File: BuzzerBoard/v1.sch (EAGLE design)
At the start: 7 parts, among them U1 LM386MX-1/NOPB

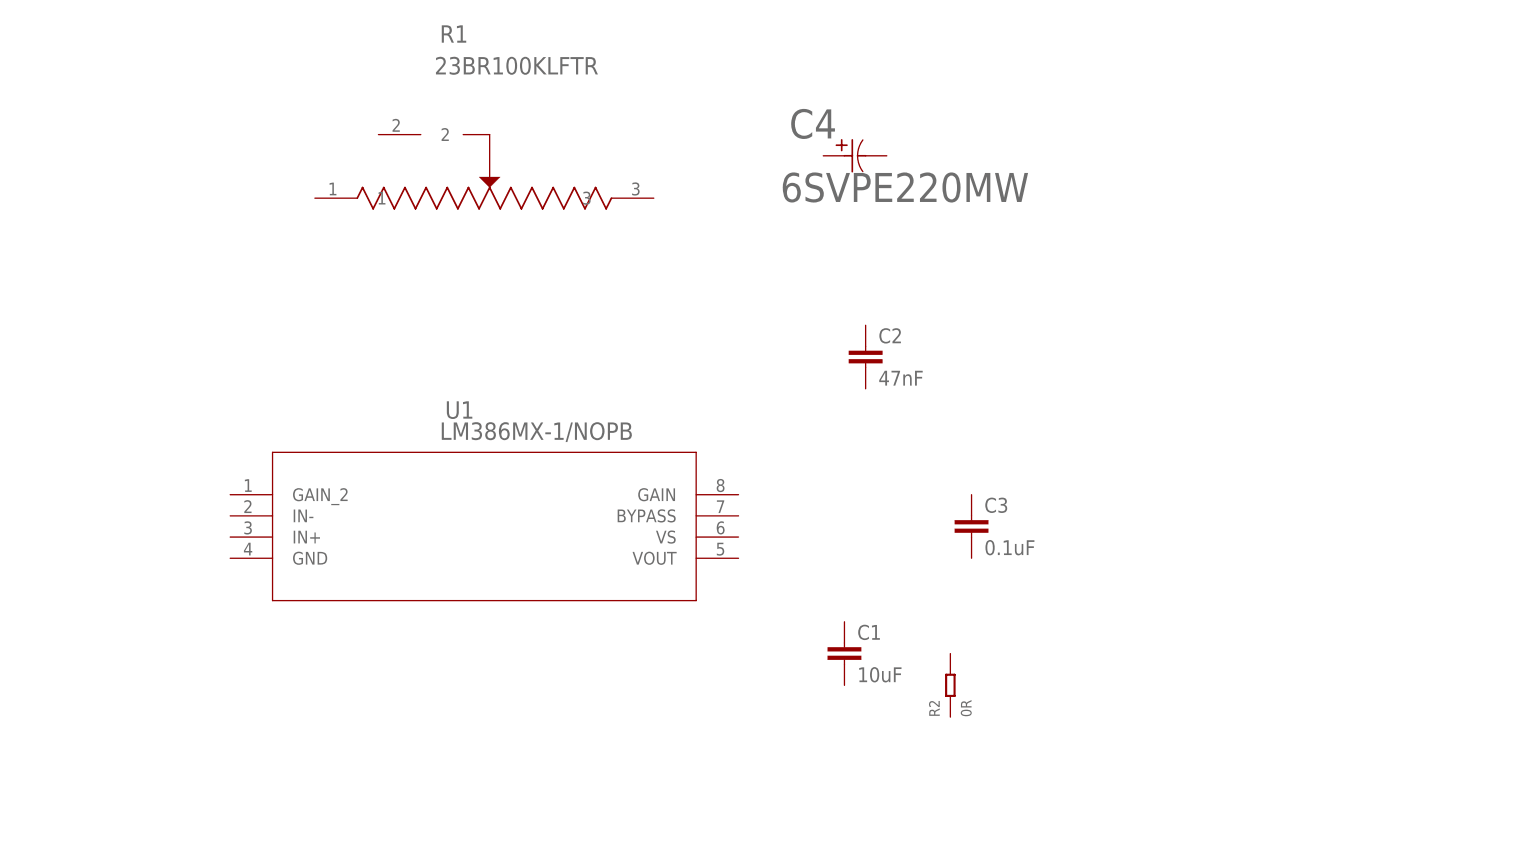
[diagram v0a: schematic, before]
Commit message: Initial schematic capture.
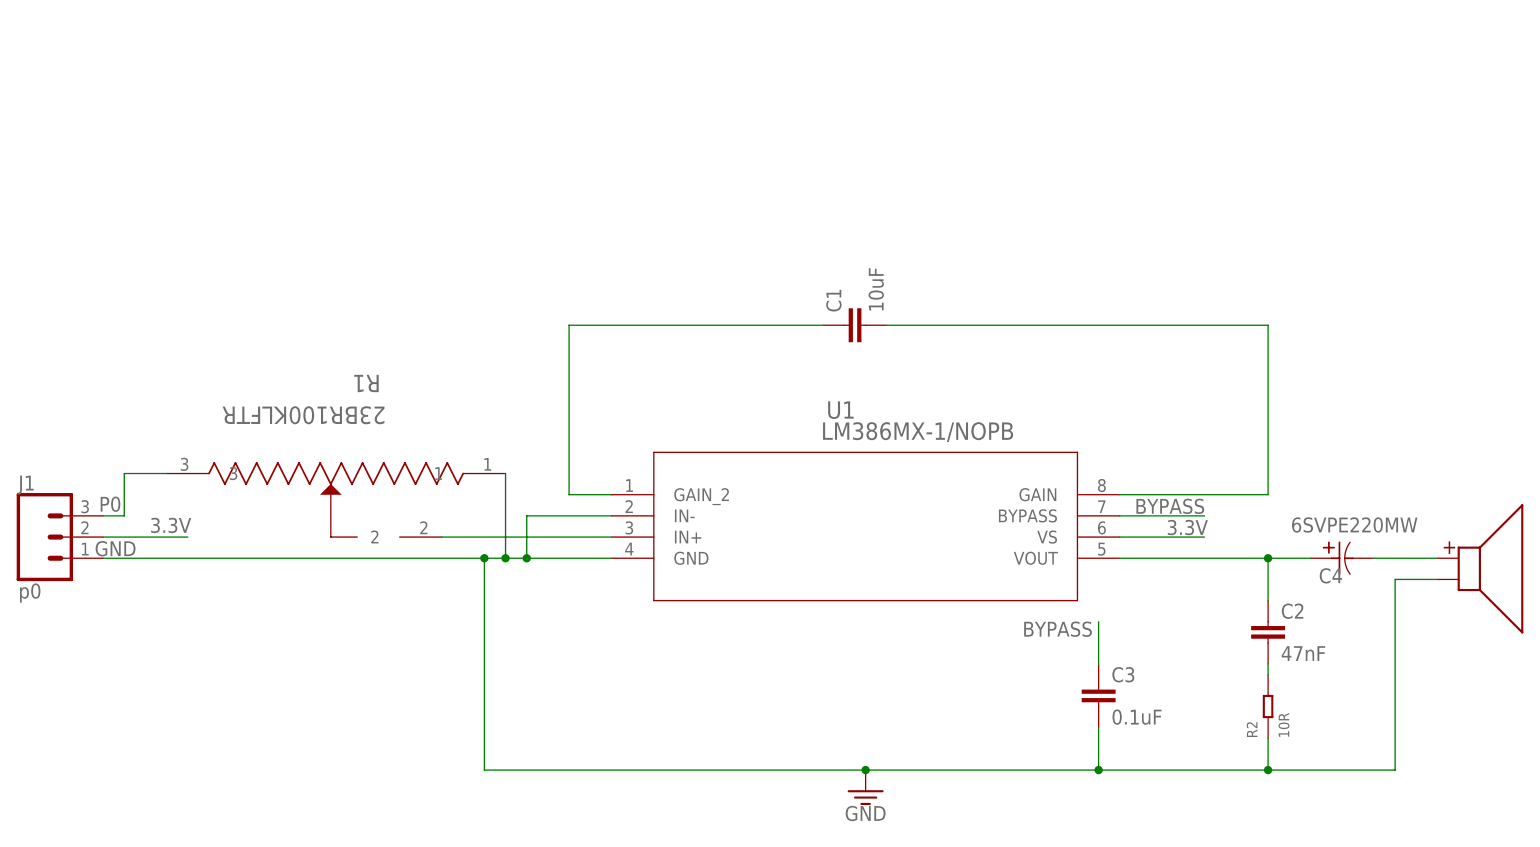
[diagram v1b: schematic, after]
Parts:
- added J1: p0, SparkFun-Connectors:CONN_03SMD_RA_MALE
- added U$1: SMS-1308MS-2-R, BuzzerLib:SMS-1308MS-2-R
- R2: value 0R -> 10R
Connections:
- new net +: C4.22, U$1.+
- new net 3.3V: J1.2, U1.VS
- new net BYPASS: C3.1, U1.BYPASS
- new net GAIN: C1.2, U1.GAIN
- new net GND: C3.2, J1.1, R1.1, R2.1, U$1.-, U1.GND, U1.IN-
- new net IN+: R1.2, U1.IN+
- new net N$1: C2.2, R2.2
- new net N$2: C1.1, U1.GAIN_2
- new net N$3: C2.1, C4.11, U1.VOUT
- new net P0: J1.3, R1.3
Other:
- moved on the sheet: C1, C2, C3, C4, R1, R2, U1
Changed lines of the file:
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@@
 <part name="C2" library="SparkFun-Capacitors" library_urn="urn:adsk.eagle:library:510" deviceset="47NF" device="-0603-25V-5%" package3d_urn="urn:adsk.eagle:package:37414/1" value="47nF"/>
 <part name="C3" library="SparkFun-Capacitors" library_urn="urn:adsk.eagle:library:510" deviceset="0.1UF" device="-0603-25V-(+80/-20%)" package3d_urn="urn:adsk.eagle:package:37414/1" value="0.1uF"/>
-<part name="R2" library="Seeed-Resistor" library_urn="urn:adsk.eagle:library:474" deviceset="SMD-RES-0R-5%-1/10W(0603)" device="" package3d_urn="urn:adsk.eagle:package:32791/1" value="0R"/>
+<part name="R2" library="Seeed-Resistor" library_urn="urn:adsk.eagle:library:474" deviceset="SMD-RES-0R-5%-1/10W(0603)" device="" package3d_urn="urn:adsk.eagle:package:32791/1" value="10R"/>
 <part name="C4" library="BuzzerLib" deviceset="6SVPE220MW" device=""/>
+<part name="U$1" library="BuzzerLib" deviceset="SMS-1308MS-2-R" device=""/>
+<part name="J1" library="SparkFun-Connectors" library_urn="urn:adsk.eagle:library:513" deviceset="CONN_03" device="SMD_RA_MALE" package3d_urn="urn:adsk.eagle:package:38078/1" value="p0"/>
+<part name="GND" library="SparkFun-PowerSymbols" library_urn="urn:adsk.eagle:library:530" deviceset="GND2" device="" value="GND"/>
 </parts>
 <sheets>
@@
 </plain>
 <instances>
-<instance part="U1" gate="A" x="5.08" y="20.32"/>
-<instance part="R1" gate="A" x="15.24" y="55.88"/>
-<instance part="C1" gate="G$1" x="81.28" y="0"/>
-<instance part="C2" gate="G$1" x="83.82" y="35.56"/>
-<instance part="C3" gate="G$1" x="96.52" y="15.24"/>
-<instance part="R2" gate="G$1" x="93.98" y="-2.54" rot="R90"/>
-<instance part="C4" gate="A" x="78.74" y="60.96"/>
+<instance part="U1" gate="A" x="50.8" y="20.32"/>
+<instance part="R1" gate="A" x="43.18" y="22.86" smashed="yes" rot="R180">
+<attribute name="VALUE" x="26.3144" y="30.8864" size="2.0828" layer="96" ratio="6" rot="SR180"/>
+<attribute name="NAME" x="25.6794" y="34.6964" size="2.0828" layer="95" ratio="6" rot="SR180"/>
+</instance>
+<instance part="C1" gate="G$1" x="83.82" y="40.64" rot="R90"/>
+<instance part="C2" gate="G$1" x="132.08" y="2.54"/>
+<instance part="C3" gate="G$1" x="111.76" y="-5.08"/>
+<instance part="R2" gate="G$1" x="132.08" y="-5.08" rot="R90"/>
+<instance part="C4" gate="A" x="137.16" y="12.7" smashed="yes">
+<attribute name="VALUE" x="134.7978" y="15.7988" size="1.778" layer="96" ratio="10" rot="SR0"/>
+<attribute name="NAME" x="138.1506" y="9.7028" size="1.778" layer="95" ratio="10" rot="SR0"/>
+</instance>
+<instance part="U$1" gate="G$1" x="154.94" y="8.89"/>
+<instance part="J1" gate="J$1" x="-15.24" y="15.24"/>
+<instance part="GND" gate="G$1" x="83.82" y="-15.24"/>
 </instances>
 <busses>
 </busses>
 <nets>
+<net name="IN+" class="0">
+<segment>
+<pinref part="R1" gate="A" pin="2"/>
+<pinref part="U1" gate="A" pin="IN+"/>
+<wire x1="33.02" y1="15.24" x2="53.34" y2="15.24" width="0.1524" layer="91"/>
+</segment>
+</net>
+<net name="P0" class="0">
+<segment>
+<pinref part="J1" gate="J$1" pin="3"/>
+<wire x1="-7.62" y1="17.78" x2="-5.08" y2="17.78" width="0.1524" layer="91"/>
+<wire x1="-5.08" y1="17.78" x2="-5.08" y2="22.86" width="0.1524" layer="91"/>
+<pinref part="R1" gate="A" pin="3"/>
+<wire x1="-5.08" y1="22.86" x2="0" y2="22.86" width="0.1524" layer="91"/>
+<label x="-8.128" y="18.288" size="1.778" layer="95"/>
+</segment>
+</net>
+<net name="3.3V" class="0">
+<segment>
+<pinref part="J1" gate="J$1" pin="2"/>
+<wire x1="-7.62" y1="15.24" x2="2.54" y2="15.24" width="0.1524" layer="91"/>
+<label x="-2.032" y="15.748" size="1.778" layer="95"/>
+</segment>
+<segment>
+<pinref part="U1" gate="A" pin="VS"/>
+<wire x1="114.3" y1="15.24" x2="124.46" y2="15.24" width="0.1524" layer="91"/>
+<label x="119.888" y="15.494" size="1.778" layer="95"/>
+</segment>
+</net>
+<net name="GND" class="0">
+<segment>
+<pinref part="U1" gate="A" pin="GND"/>
+<wire x1="-7.62" y1="12.7" x2="38.1" y2="12.7" width="0.1524" layer="91"/>
+<pinref part="J1" gate="J$1" pin="1"/>
+<wire x1="38.1" y1="12.7" x2="40.64" y2="12.7" width="0.1524" layer="91"/>
+<wire x1="40.64" y1="12.7" x2="43.18" y2="12.7" width="0.1524" layer="91"/>
+<wire x1="43.18" y1="12.7" x2="53.34" y2="12.7" width="0.1524" layer="91"/>
+<pinref part="R1" gate="A" pin="1"/>
+<wire x1="40.64" y1="22.86" x2="40.64" y2="12.7" width="0.1524" layer="91"/>
+<junction x="40.64" y="12.7"/>
+<pinref part="U1" gate="A" pin="IN-"/>
+<wire x1="53.34" y1="17.78" x2="43.18" y2="17.78" width="0.1524" layer="91"/>
+<wire x1="43.18" y1="17.78" x2="43.18" y2="12.7" width="0.1524" layer="91"/>
+<junction x="43.18" y="12.7"/>
+<pinref part="GND" gate="G$1" pin="3.3V"/>
+<wire x1="83.82" y1="-12.7" x2="38.1" y2="-12.7" width="0.1524" layer="91"/>
+<wire x1="38.1" y1="-12.7" x2="38.1" y2="12.7" width="0.1524" layer="91"/>
+<junction x="38.1" y="12.7"/>
+<label x="-8.636" y="12.954" size="1.778" layer="95"/>
+<wire x1="83.82" y1="-12.7" x2="111.76" y2="-12.7" width="0.1524" layer="91"/>
+<wire x1="111.76" y1="-12.7" x2="132.08" y2="-12.7" width="0.1524" layer="91"/>
+<wire x1="132.08" y1="-12.7" x2="147.32" y2="-12.7" width="0.1524" layer="91"/>
+<wire x1="147.32" y1="-12.7" x2="147.32" y2="10.16" width="0.1524" layer="91"/>
+<junction x="83.82" y="-12.7"/>
+<pinref part="U$1" gate="G$1" pin="-"/>
+<wire x1="147.32" y1="10.16" x2="152.4" y2="10.16" width="0.1524" layer="91"/>
+<pinref part="C3" gate="G$1" pin="2"/>
+<wire x1="111.76" y1="-7.62" x2="111.76" y2="-12.7" width="0.1524" layer="91"/>
+<junction x="111.76" y="-12.7"/>
+<pinref part="R2" gate="G$1" pin="1"/>
+<wire x1="132.08" y1="-8.89" x2="132.08" y2="-12.7" width="0.1524" layer="91"/>
+<junction x="132.08" y="-12.7"/>
+</segment>
+</net>
+<net name="+" class="0">
+<segment>
+<pinref part="C4" gate="A" pin="22"/>
+<pinref part="U$1" gate="G$1" pin="+"/>
+<wire x1="144.78" y1="12.7" x2="152.4" y2="12.7" width="0.1524" layer="91"/>
+</segment>
+</net>
+<net name="GAIN" class="0">
+<segment>
+<pinref part="U1" gate="A" pin="GAIN"/>
+<wire x1="132.08" y1="20.32" x2="114.3" y2="20.32" width="0.1524" layer="91"/>
+<pinref part="C1" gate="G$1" pin="2"/>
+<wire x1="86.36" y1="40.64" x2="132.08" y2="40.64" width="0.1524" layer="91"/>
+<wire x1="132.08" y1="40.64" x2="132.08" y2="20.32" width="0.1524" layer="91"/>
+</segment>
+</net>
+<net name="BYPASS" class="0">
+<segment>
+<pinref part="C3" gate="G$1" pin="1"/>
+<wire x1="111.76" y1="0" x2="111.76" y2="5.08" width="0.1524" layer="91"/>
+<label x="102.616" y="3.302" size="1.778" layer="95"/>
+</segment>
+<segment>
+<pinref part="U1" gate="A" pin="BYPASS"/>
+<wire x1="114.3" y1="17.78" x2="124.46" y2="17.78" width="0.1524" layer="91"/>
+<label x="116.078" y="18.034" size="1.778" layer="95"/>
+</segment>
+</net>
+<net name="N$1" class="0">
+<segment>
+<pinref part="R2" gate="G$1" pin="2"/>
+<pinref part="C2" gate="G$1" pin="2"/>
+<wire x1="132.08" y1="-1.27" x2="132.08" y2="0" width="0.1524" layer="91"/>
+</segment>
+</net>
+<net name="N$2" class="0">
+<segment>
+<pinref part="U1" gate="A" pin="GAIN_2"/>
+<wire x1="53.34" y1="20.32" x2="48.26" y2="20.32" width="0.1524" layer="91"/>
+<wire x1="48.26" y1="20.32" x2="48.26" y2="40.64" width="0.1524" layer="91"/>
+<pinref part="C1" gate="G$1" pin="1"/>
+<wire x1="48.26" y1="40.64" x2="78.74" y2="40.64" width="0.1524" layer="91"/>
+</segment>
+</net>
+<net name="N$3" class="0">
+<segment>
+<pinref part="C4" gate="A" pin="11"/>
+<wire x1="137.16" y1="12.7" x2="132.08" y2="12.7" width="0.1524" layer="91"/>
+<pinref part="C2" gate="G$1" pin="1"/>
+<wire x1="132.08" y1="7.62" x2="132.08" y2="12.7" width="0.1524" layer="91"/>
+<pinref part="U1" gate="A" pin="VOUT"/>
+<wire x1="114.3" y1="12.7" x2="132.08" y2="12.7" width="0.1524" layer="91"/>
+<junction x="132.08" y="12.7"/>
+</segment>
+</net>
 </nets>
 </sheet>
 </sheets>
+<errors>
+</errors>
 </schematic>
 </drawing>

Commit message: V1 to OSH park.
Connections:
- net N$3 renamed VOUT
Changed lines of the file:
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@@
 </segment>
 </net>
-<net name="N$3" class="0">
+<net name="VOUT" class="0">
 <segment>
 <pinref part="C4" gate="A" pin="11"/>
